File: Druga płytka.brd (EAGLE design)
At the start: 26.2 x 25.6 mm, 6 parts, among them J1 826629-8, U1 MB85RS64V, U2 SCD40-D-R1

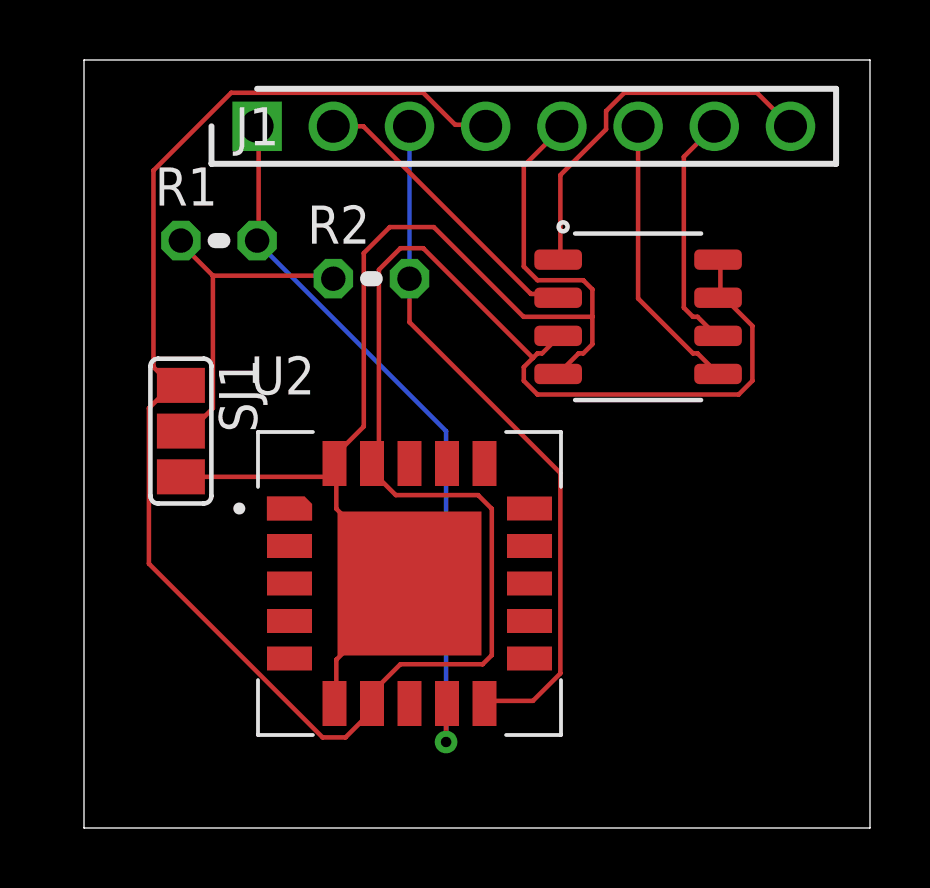
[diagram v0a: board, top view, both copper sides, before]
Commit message: Add final project of PCB boards and cleaning repository up
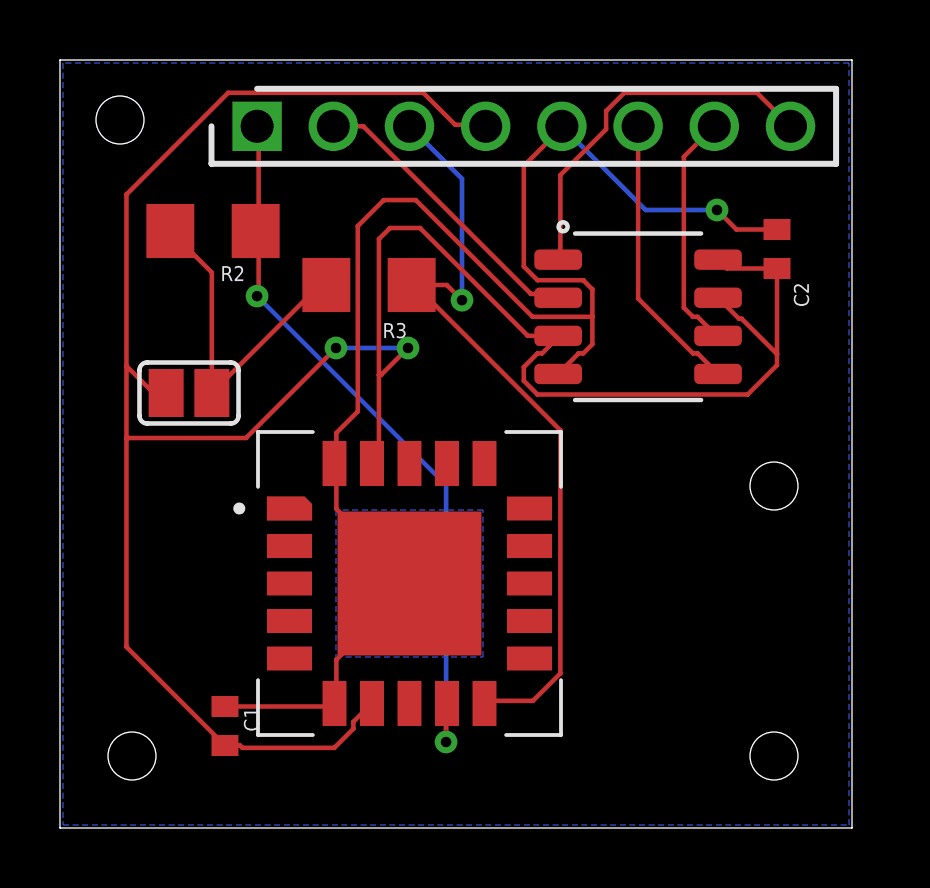
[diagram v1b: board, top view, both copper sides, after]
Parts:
- removed R1: 1k, rcl:0204V
- removed SJ1: (no value), jumper:SJ_2
- added C1, C2: 100nF, rcl:C0402
- added R3: 4k7, rcl:R1206
- added SJ2: (no value), jumper:SJ
- R2: value 1k -> 4k7; device rcl:0204V -> rcl:R1206
- moved R2 5.51 mm to (-22.7, 21.1), turned to 180 degrees
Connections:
- net 3V3: now also C1.2, C2.1, SJ2.1; no longer SJ1.1
- net GND: now also C1.1, C2.2; no longer SJ1.3
- net JUMPER: now also R2.2, R3.2, SJ2.2; no longer R1.1, R2.1, SJ1.2
- net SCL: now also R2.1; no longer R1.2
- net SDA: now also R3.1; no longer R2.2
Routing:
- net 3V3: track 79.9 -> 88.4 mm, vias 0 -> 2
- net GND: track 43.5 -> 52.0 mm, vias 0 -> 1
- net SDA: track 23.3 -> 26.4 mm, vias 0 -> 1
- net SCL: track 24.4 -> 24.5 mm, vias 1 -> 2
- added copper zone on layer 16, net GND
- added copper zone on layer 16, net NONE
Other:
- board size 26.2 x 25.6 mm -> 26.4 x 25.6 mm
